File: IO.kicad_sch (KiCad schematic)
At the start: 22 parts, among them P14 14.31818 MHz CLK, P53 FRONT_PANEL, U15 74LS245, U16 74LS244, U18 74LS32, U27 74LS245, U28 74LS245, U4 74LS245, U6 74LS32

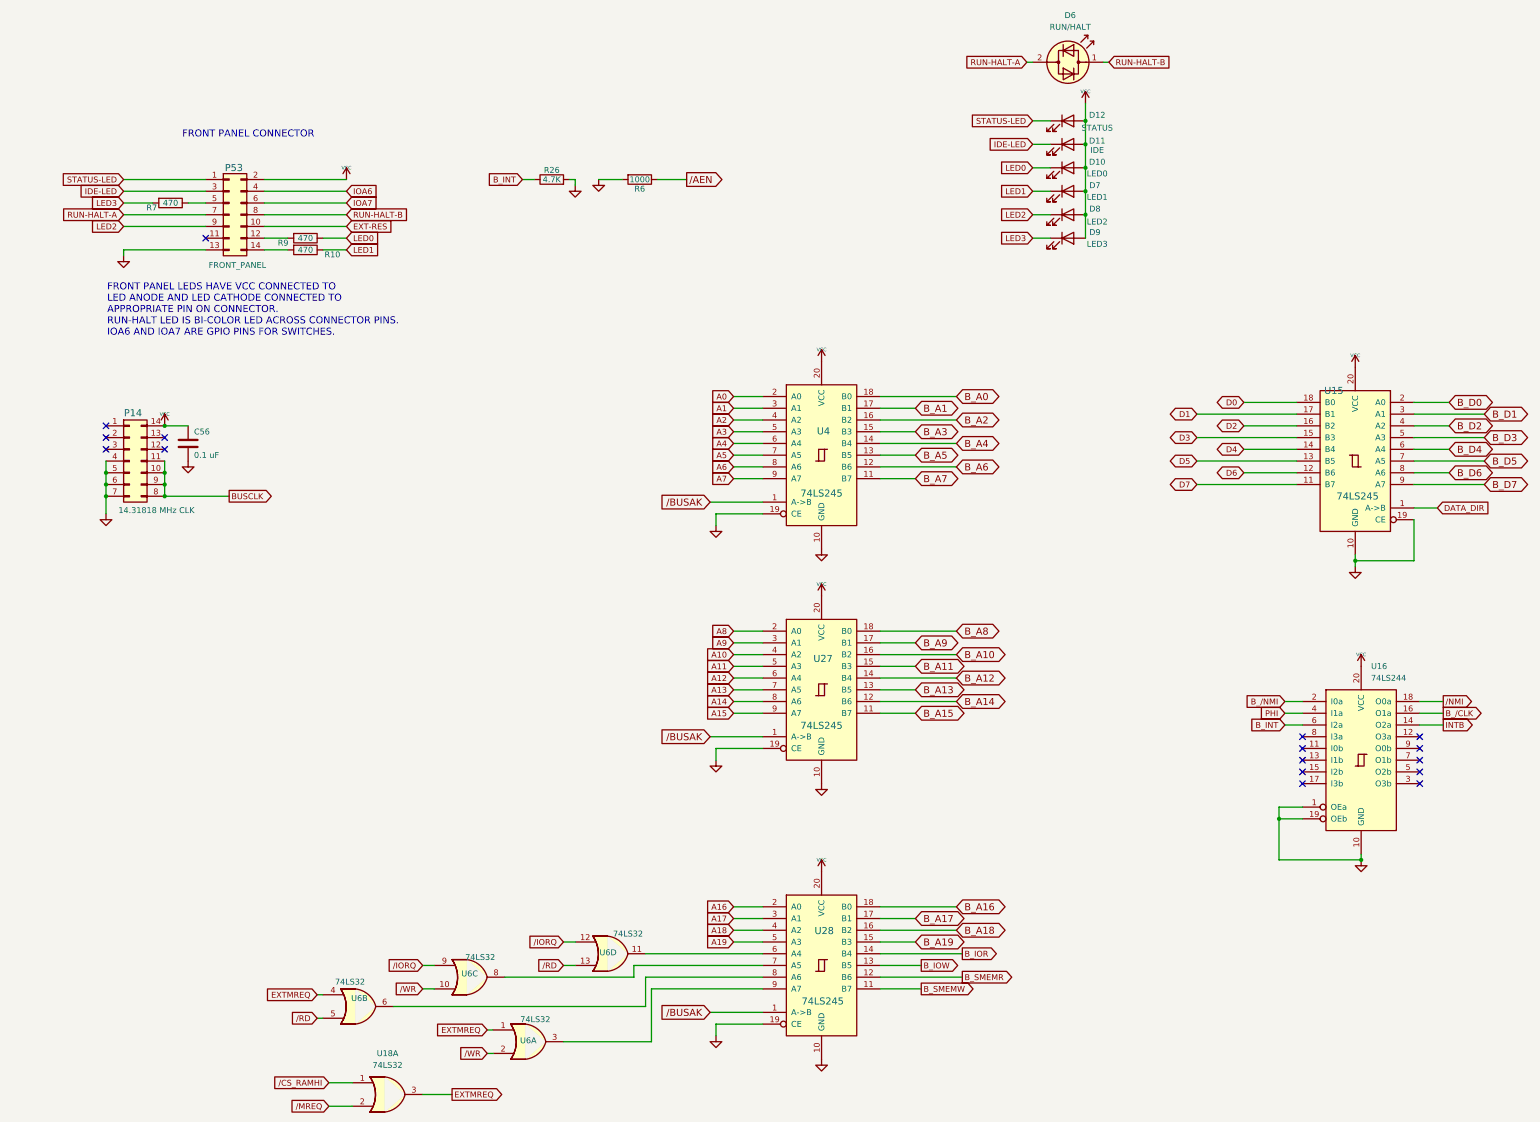
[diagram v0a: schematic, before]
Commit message: rev 1.0
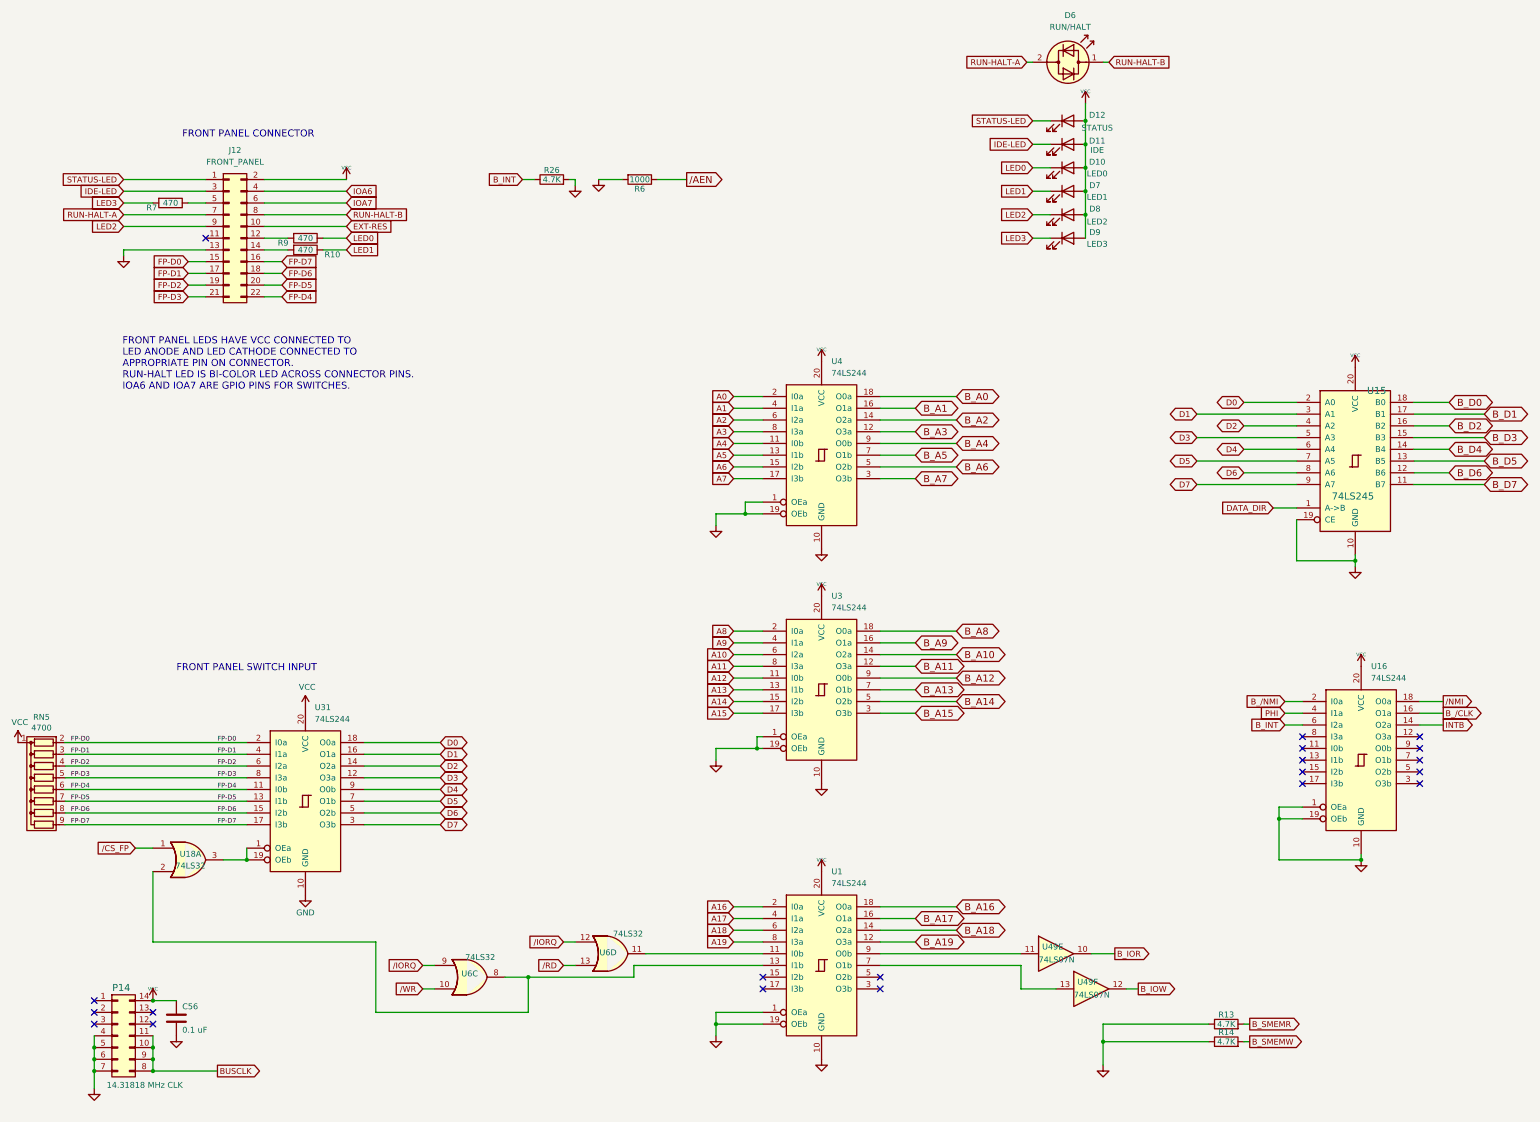
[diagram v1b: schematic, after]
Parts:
- removed P53: FRONT_PANEL, Custom:STD_DDW_PinHeader_2x07, symbol Connector_Generic:Conn_02x07_Odd_Even
- removed U27, U28, U4: 74LS245, Custom:STD_DDW_DIP20, symbol 74xx:74LS245
- removed unit 1 of U6
- removed unit 2 of U6
- added J12: FRONT_PANEL, Custom:STD_DDW_PinHeader_2x11, symbol Connector_Generic:Conn_02x11_Odd_Even
- added R13, R14: 4.7K, Custom:STD_DDW_RESISTOR, symbol Device:R
- added RN5: 4700, Resistor_THT:R_Array_SIP9, symbol Device:R_Network08
- added U1, U3, U31, U4: 74LS244, Custom:STD_DDW_DIP20, symbol 74xx:74LS244
- added U49: 74LS07N, Custom:STD_DDW_DIP14, symbol 74xx:74LS07
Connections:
- net /MREQ is gone; now on an unnamed net: U18.2
- net A0: now also U4.2 (I0a)
- net A1: now also U4.4 (I1a)
- net A10: now also U3.6 (I2a)
- net A11: now also U3.8 (I3a)
- net A12: now also U3.11 (I0b)
- net A13: now also U3.13 (I1b)
- net A14: now also U3.15 (I2b)
- net A15: now also U3.17 (I3b)
- net A16: now also U1.2 (I0a)
- net A17: now also U1.4 (I1a)
- net A18: now also U1.6 (I2a)
- net A19: now also U1.8 (I3a)
- net A2: now also U4.6 (I2a)
- net A3: now also U4.8 (I3a)
- net A4: now also U4.11 (I0b)
- net A5: now also U4.13 (I1b)
- net A6: now also U4.15 (I2b)
- net A7: now also U4.17 (I3b)
- net A8: now also U3.2 (I0a)
- net A9: now also U3.4 (I1a)
- net B_A0: now also U4.18 (O0a)
- net B_A1: now also U4.16 (O1a)
- net B_A10: now also U3.14 (O2a)
- net B_A11: now also U3.12 (O3a)
- net B_A12: now also U3.9 (O0b)
- net B_A13: now also U3.7 (O1b)
- net B_A14: now also U3.5 (O2b)
- net B_A15: now also U3.3 (O3b)
- net B_A16: now also U1.18 (O0a)
- net B_A17: now also U1.16 (O1a)
- net B_A18: now also U1.14 (O2a)
- net B_A19: now also U1.12 (O3a)
- net B_A2: now also U4.14 (O2a)
- net B_A3: now also U4.12 (O3a)
- net B_A4: now also U4.9 (O0b)
- net B_A5: now also U4.7 (O1b)
- net B_A6: now also U4.5 (O2b)
- net B_A7: now also U4.3 (O3b)
- net B_A8: now also U3.18 (O0a)
- net B_A9: now also U3.16 (O1a)
- net B_D0: now also U15.18 (B0); no longer U15.2 (A0)
- net B_D1: now also U15.17 (B1); no longer U15.3 (A1)
- net B_D2: now also U15.16 (B2); no longer U15.4 (A2)
- net B_D3: now also U15.15 (B3); no longer U15.5 (A3)
- net B_D4: now also U15.14 (B4); no longer U15.6 (A4)
- net B_D5: now also U15.13 (B5); no longer U15.7 (A5)
- net B_D6: now also U15.12 (B6); no longer U15.8 (A6)
- net B_D7: now also U15.11 (B7); no longer U15.9 (A7)
- net B_IOR: now also U49.10
- net B_IOW: now also U49.12
- net B_SMEMR: now also R13.2
- net B_SMEMW: now also R14.2
- net D0: now also U15.2 (A0), U31.18 (O0a); no longer U15.18 (B0)
- net D1: now also U15.3 (A1), U31.16 (O1a); no longer U15.17 (B1)
- net D2: now also U15.4 (A2), U31.14 (O2a); no longer U15.16 (B2)
- net D3: now also U15.5 (A3), U31.12 (O3a); no longer U15.15 (B3)
- net D4: now also U15.6 (A4), U31.9 (O0b); no longer U15.14 (B4)
- net D5: now also U15.7 (A5), U31.7 (O1b); no longer U15.13 (B5)
- net D6: now also U15.8 (A6), U31.5 (O2b); no longer U15.12 (B6)
- net D7: now also U15.9 (A7), U31.3 (O3b); no longer U15.11 (B7)
- net EXT-RES: now also J12.10 (Pin_10)
- net GND: now also J12.13 (Pin_13), R13.1, R14.1, U1.1 (OEa), U1.10 (GND), U1.19 (OEb), U3.1 (OEa), U3.10 (GND), U3.19 (OEb), U31.10 (GND), U4.1 (OEa), U4.10 (GND), U4.19 (OEb)
- net IDE-LED: now also J12.3 (Pin_3)
- net IOA6: now also J12.4 (Pin_4)
- net IOA7: now also J12.6 (Pin_6)
- net LED2: now also J12.9 (Pin_9)
- net RUN-HALT-A: now also J12.7 (Pin_7)
- net RUN-HALT-B: now also J12.8 (Pin_8)
- net STATUS-LED: now also J12.1 (Pin_1)
- net VCC: now also J12.2 (Pin_2), RN5.1 (common), U1.20 (VCC), U3.20 (VCC), U31.20 (VCC), U4.20 (VCC)
- net at R9.2: now also J12.12 (Pin_12)
- net at R10.2: now also J12.14 (Pin_14)
- net at R7.1: now also J12.5 (Pin_5)
- net at U6.11: now also U1.11 (I0b)
- net at U6.8: now also U1.13 (I1b)
- net EXTMREQ: no longer names the net of U18.3
- net EXTMREQ: now also U31.1 (OEa), U31.19 (OEb)
- net /CS_RAMHI renamed /CS_FP
- new net: U1.7 (O1b), U49.13
- new net: U1.9 (O0b), U49.11
- new net FP-D0: J12.15 (Pin_15), RN5.2 (R1), U31.2 (I0a)
- new net FP-D1: J12.17 (Pin_17), RN5.3 (R2), U31.4 (I1a)
- new net FP-D2: J12.19 (Pin_19), RN5.4 (R3), U31.6 (I2a)
- new net FP-D3: J12.21 (Pin_21), RN5.5 (R4), U31.8 (I3a)
- new net FP-D4: J12.22 (Pin_22), RN5.6 (R5), U31.11 (I0b)
- new net FP-D5: J12.20 (Pin_20), RN5.7 (R6), U31.13 (I1b)
- new net FP-D6: J12.18 (Pin_18), RN5.8 (R7), U31.15 (I2b)
- new net FP-D7: J12.16 (Pin_16), RN5.9 (R8), U31.17 (I3b)
- no-connect marks 16 -> 20
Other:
- note added: "FRONT PANEL SWITCH INPUT"
- moved on the sheet: C56, P14
